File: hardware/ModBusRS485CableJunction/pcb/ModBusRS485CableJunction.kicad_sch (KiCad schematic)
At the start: 5 parts, among them J1 215877-1, J2 Modbus Stub

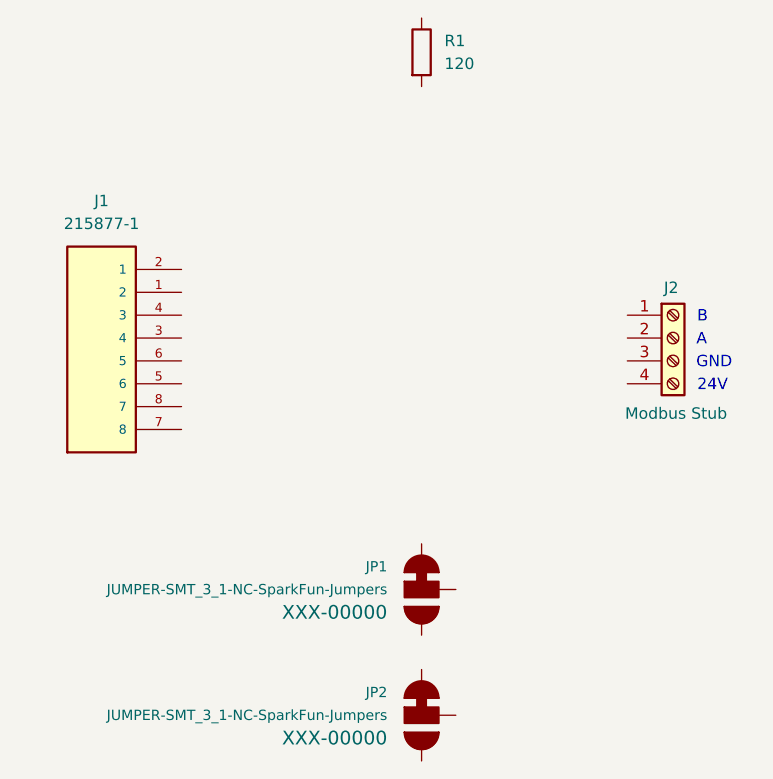
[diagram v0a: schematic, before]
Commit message: last commit of the day.
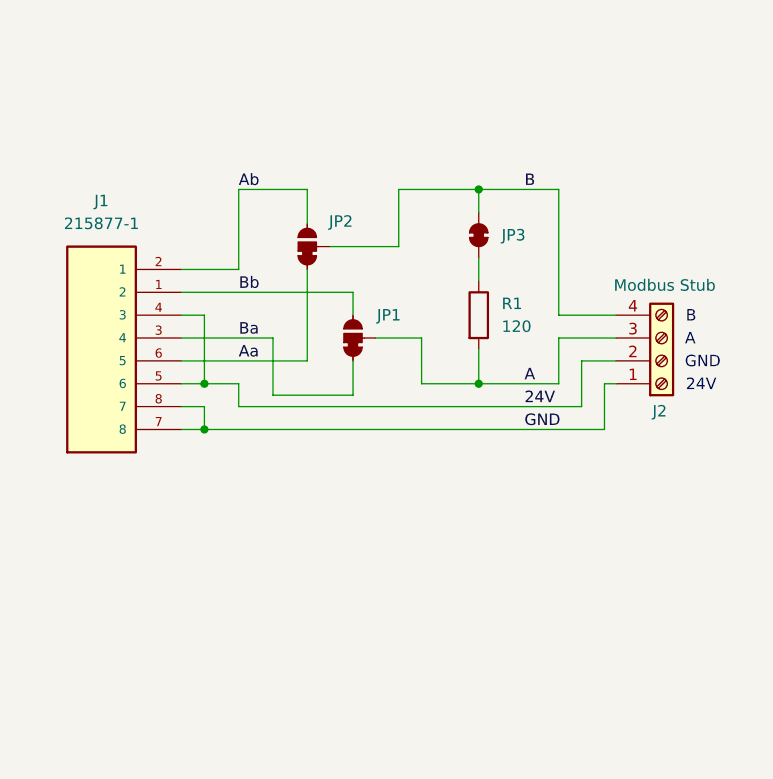
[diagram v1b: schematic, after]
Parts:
- removed JP1, JP2: JUMPER-SMT_3_1-NC-SparkFun-Jumpers, SMT-JUMPER_3_1-NC, symbol my-KiCad-library:JUMPER-SMT_3_1-NC-SparkFun-Jumpers
- added JP1, JP2: (no value), SparkFun-Jumper:Jumper_3_NC-1_Trace, symbol SparkFun-Jumper:SolderJumper_3_Bridged12
- added JP3: (no value), SparkFun-Jumper:Jumper_2_NC_Trace, symbol SparkFun-Jumper:SolderJumper_2_Bridged
- J1: footprint 215877-1:CONN_215877-1 -> my-KiCad-library:CONN_215877-1
- J2: footprint (none) -> TerminalBlock_Phoenix:TerminalBlock_Phoenix_MKDS-3-4-5.08_1x04_P5.08mm_Horizontal
- R1: footprint (none) -> Resistor_SMD:R_1206_3216Metric_Pad1.30x1.75mm_HandSolder
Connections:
- net GND: now reaches J2.1 (Pin_1)
- net GND: now also J1.7 (8), J1.8 (7)
- net 24V: now reaches J2.2 (Pin_2)
- net 24V: now also J1.4 (3), J1.5 (6)
- net A: now reaches J2.3 (Pin_3)
- net A: now also R1.2, JP1.2 (B)
- net B: now reaches J2.4 (Pin_4)
- net B: now also JP2.2 (B), JP3.2 (B)
- net Bb: now reaches J1.1 (2)
- net Bb: now also JP1.3 (C)
- net Ab: now reaches J1.2 (1)
- net Ab: now also JP2.3 (C)
- net Ba: now reaches J1.3 (4)
- net Ba: now also JP1.1 (A)
- net Aa: now reaches J1.6 (5)
- net Aa: now also JP2.1 (A)
- net at R1.1: now also JP3.1 (A)
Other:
- moved on the sheet: R1
